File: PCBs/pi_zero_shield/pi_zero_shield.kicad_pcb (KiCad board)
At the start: 2 copper layers, 30.8 x 65 mm, 3 parts, among them J1 T1M-10-F-SH-L-K, J2 Conn_02x20_Odd_Even, J3 T1M-06-X-DV

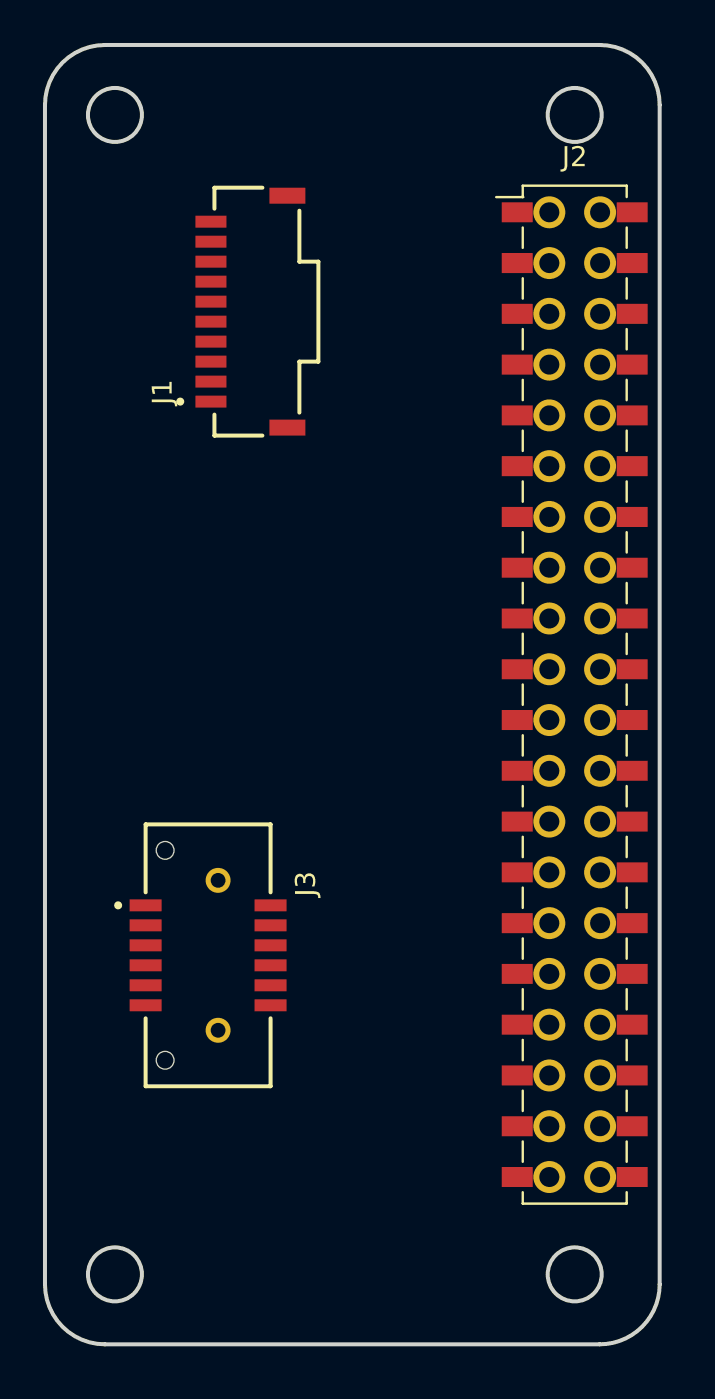
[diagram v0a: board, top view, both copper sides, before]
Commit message: number of PCBs for 2nd round of Maka Niu fabrication, in their state after orders made.
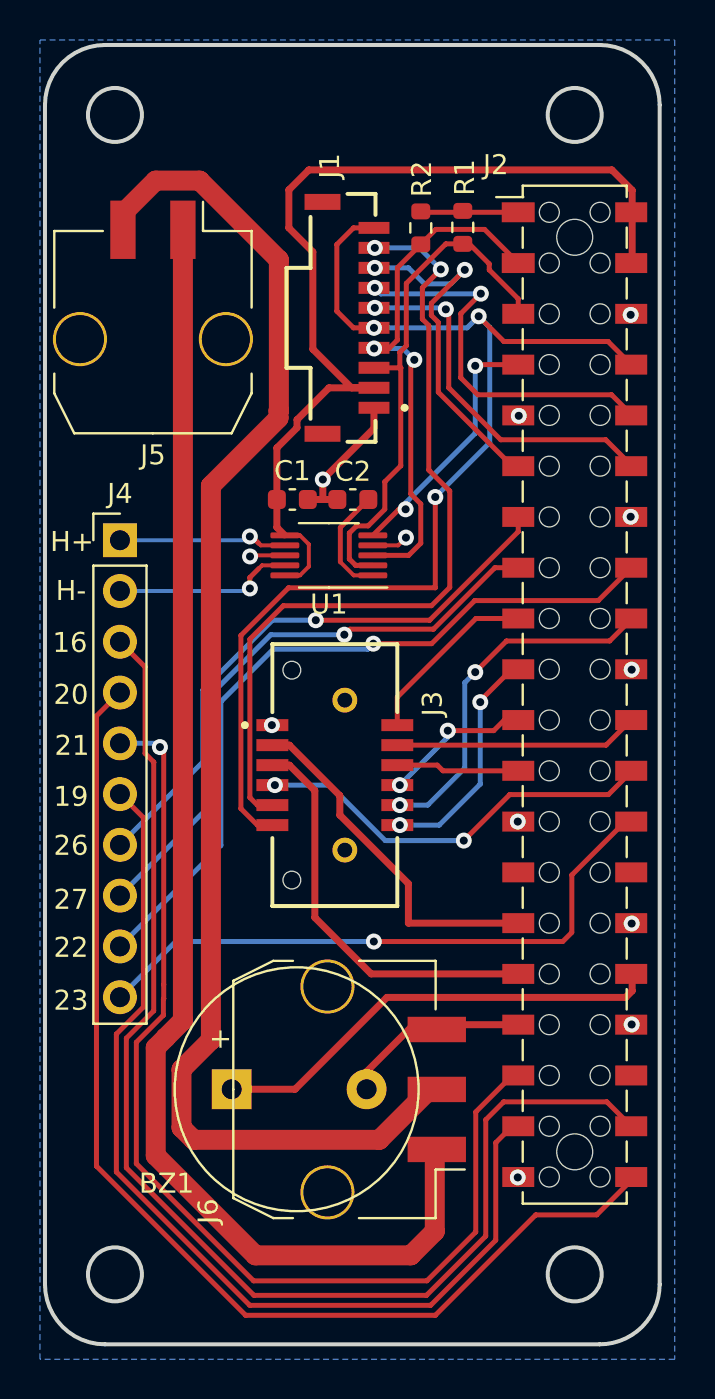
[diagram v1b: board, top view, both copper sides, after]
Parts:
- added BZ1: Buzzer, custom:Buzzer_12x9.5RM7.6, F.Cu at (126.6, 125.5)
- added C1: 1.0uF, Capacitor_SMD:C_0603_1608Metric, F.Cu at (126.4, 96.0)
- added C2: 1.0uF, Capacitor_SMD:C_0603_1608Metric, F.Cu at (129.4, 96.0)
- added J4: Screw_Terminal_01x10, Connector_PinHeader_2.54mm:PinHeader_1x10_P2.54mm_Vertical, F.Cu at (117.8, 98.0)
- added J5: Conn_01x02, Connector_Molex:Molex_Micro-Fit_3.0_43650-0210_1x02-1MP_P3.00mm_Horizontal, F.Cu at (119.4, 87.6)
- added J6: Conn_01x03, Connector_Molex:Molex_Micro-Fit_3.0_43650-0310_1x03-1MP_P3.00mm_Horizontal, F.Cu at (128.5, 125.5)
- added R1: 10K, Resistor_SMD:R_0603_1608Metric, F.Cu at (134.9, 82.4)
- added R2: 10K, Resistor_SMD:R_0603_1608Metric, F.Cu at (132.8, 82.4)
- added U1: DRV2605LDGS, Package_SO:VSSOP-10_3x3mm_P0.5mm, F.Cu at (128.2, 98.8)
- J1: value T1M-10-F-SH-L-K -> T1M-10-F-SV-L; footprint custom:SAMTEC_T1M-10-F-SH-L-K -> custom:SAMTEC_T1M-10-F-SV-L
- moved J3 11.0 mm to (128.5, 109.8)
- moved J1 8.16 mm to (130.5, 86.9)
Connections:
- J2 pad 1: unconnected-(J2-Pad1) -> /3.3V pullup
- J2 pad 10: unconnected-(J2-Pad10) -> GPS_INT
- J2 pad 11: unconnected-(J2-Pad11) -> IMU_INT
- J2 pad 12: unconnected-(J2-Pad12) -> ENDCAP_EN
- J2 pad 13: unconnected-(J2-Pad13) -> GPIO27
- J2 pad 14: unconnected-(J2-Pad14) -> GND
- J2 pad 15: unconnected-(J2-Pad15) -> GPIO22
- J2 pad 16: unconnected-(J2-Pad16) -> GPIO23
- J2 pad 17: unconnected-(J2-Pad17) -> +3.3VP
- J2 pad 18: unconnected-(J2-Pad18) -> Hall_M2
- J2 pad 19: unconnected-(J2-Pad19) -> Hall_M1
- J2 pad 2: unconnected-(J2-Pad2) -> +5V
- J2 pad 20: unconnected-(J2-Pad20) -> GND
- J2 pad 21: unconnected-(J2-Pad21) -> Hall_Image
- J2 pad 22: unconnected-(J2-Pad22) -> Hall_Video
- J2 pad 23: unconnected-(J2-Pad23) -> Hall_Wifi
- J2 pad 24: unconnected-(J2-Pad24) -> Hall_Button
- J2 pad 25: unconnected-(J2-Pad25) -> GND
- J2 pad 26: unconnected-(J2-Pad26) -> GPIO17
- J2 pad 29: unconnected-(J2-Pad29) -> Green_LED
- J2 pad 3: unconnected-(J2-Pad3) -> SDA
- J2 pad 30: unconnected-(J2-Pad30) -> GND
- J2 pad 31: unconnected-(J2-Pad31) -> Red_LED
- J2 pad 32: unconnected-(J2-Pad32) -> Net-(BZ1-Pad1)
- J2 pad 33: unconnected-(J2-Pad33) -> /PWM_13
- J2 pad 34: unconnected-(J2-Pad34) -> GND
- J2 pad 35: unconnected-(J2-Pad35) -> GPIO19
- J2 pad 37: unconnected-(J2-Pad37) -> GPIO26
- J2 pad 38: unconnected-(J2-Pad38) -> GPIO20
- J2 pad 39: unconnected-(J2-Pad39) -> GND
- J2 pad 4: unconnected-(J2-Pad4) -> +5V
- J2 pad 40: unconnected-(J2-Pad40) -> GPIO21
- J2 pad 5: unconnected-(J2-Pad5) -> SCL
- J2 pad 6: unconnected-(J2-Pad6) -> GND
- J2 pad 7: unconnected-(J2-Pad7) -> Haptic_EN
- J2 pad 8: unconnected-(J2-Pad8) -> ~{SHUT_DWN_SIG}
- J2 pad 9: unconnected-(J2-Pad9) -> GND
- J3 pad 01: unconnected-(J3-Pad01) -> GND
- J3 pad 02: unconnected-(J3-Pad02) -> +3.3VP
- J3 pad 03: unconnected-(J3-Pad03) -> Green_LED
- J3 pad 04: unconnected-(J3-Pad04) -> Hall_Video
- J3 pad 05: unconnected-(J3-Pad05) -> Red_LED
- J3 pad 06: unconnected-(J3-Pad06) -> Hall_Wifi
- J3 pad 07: unconnected-(J3-Pad07) -> Hall_Button
- J3 pad 08: unconnected-(J3-Pad08) -> Hall_Image
- J3 pad 09: unconnected-(J3-Pad09) -> +3V3
- J3 pad 10: unconnected-(J3-Pad10) -> Hall_M2
- J3 pad 11: unconnected-(J3-Pad11) -> ~{SHUT_DWN_SIG}
- J3 pad 12: unconnected-(J3-Pad12) -> Hall_M1
- J3 pad S2: unconnected-(J3-PadS1) -> unconnected-(J3-PadS2)
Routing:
- net GNDPWR: track 0.00 -> 70.1 mm
- net +12V: track 0.00 -> 67.5 mm
- net GPIO20: track 0.00 -> 63.4 mm
- net ~{SHUT_DWN_SIG}: track 0.00 -> 58.1 mm, vias 0 -> 3
- net GPIO21: track 0.00 -> 57.0 mm
- net GPIO19: track 0.00 -> 52.9 mm, vias 0 -> 1
- net GPIO26: track 0.00 -> 49.4 mm
- net +5V: track 0.00 -> 48.7 mm
- net +3V3: track 0.00 -> 40.9 mm, vias 0 -> 2
- net GPIO23: track 0.00 -> 37.6 mm, vias 0 -> 1
- net GPIO17: track 0.00 -> 30.9 mm, vias 0 -> 1
- net GPIO22: track 0.00 -> 29.9 mm, vias 0 -> 1
- net GPIO27: track 0.00 -> 29.3 mm, vias 0 -> 1
- net SDA: track 0.00 -> 26.9 mm, vias 0 -> 2
- net SCL: track 0.00 -> 26.5 mm
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- added copper zone on B.Cu, net GND
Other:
- board text added: "16"
- board text added: "19"
- board text added: "20"
- board text added: "21"
- board text added: "22"
- board text added: "23"
- board text added: "26"
- board text added: "27"
- board text added: "H+"
- board text added: "H-"
